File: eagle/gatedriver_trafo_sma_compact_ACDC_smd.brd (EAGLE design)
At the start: 108 x 108 mm, 60 parts, among them K1 G5V-2, X4 BU-SMA-V

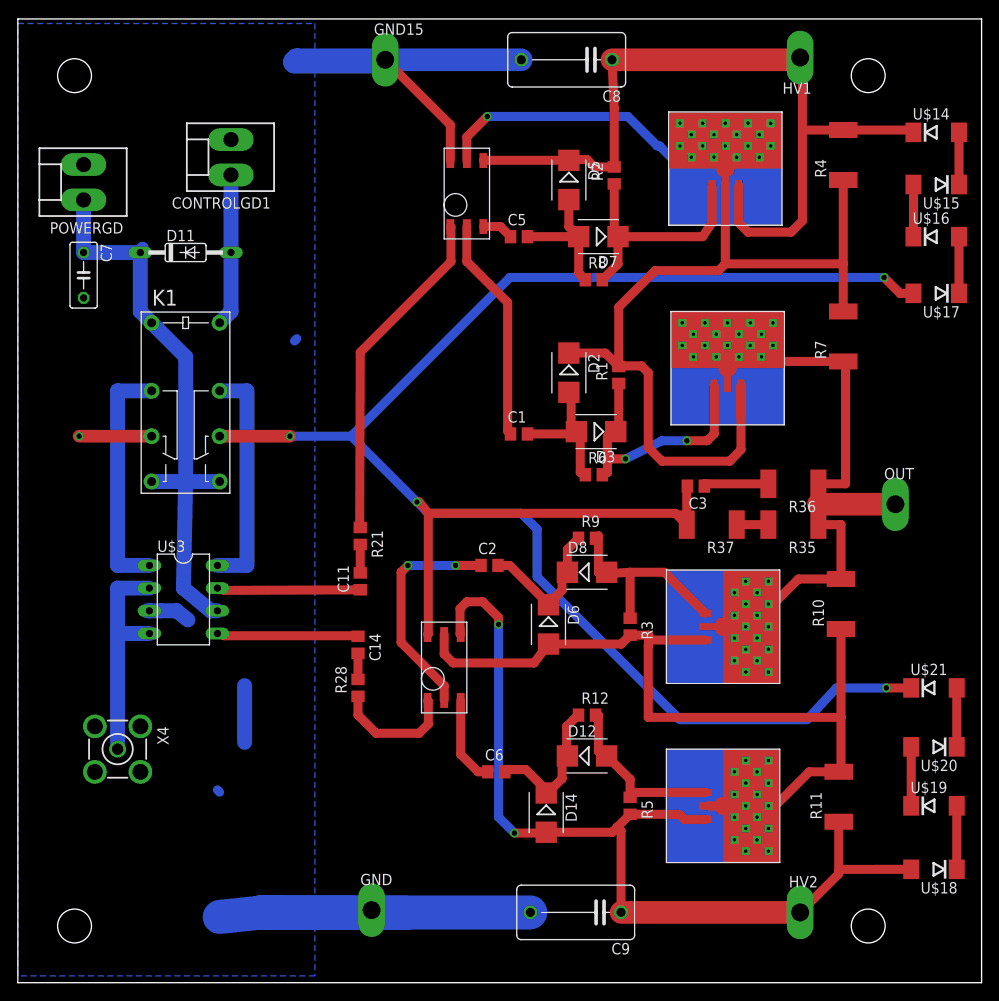
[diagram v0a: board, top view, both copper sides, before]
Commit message: Heatsink, CTIA code
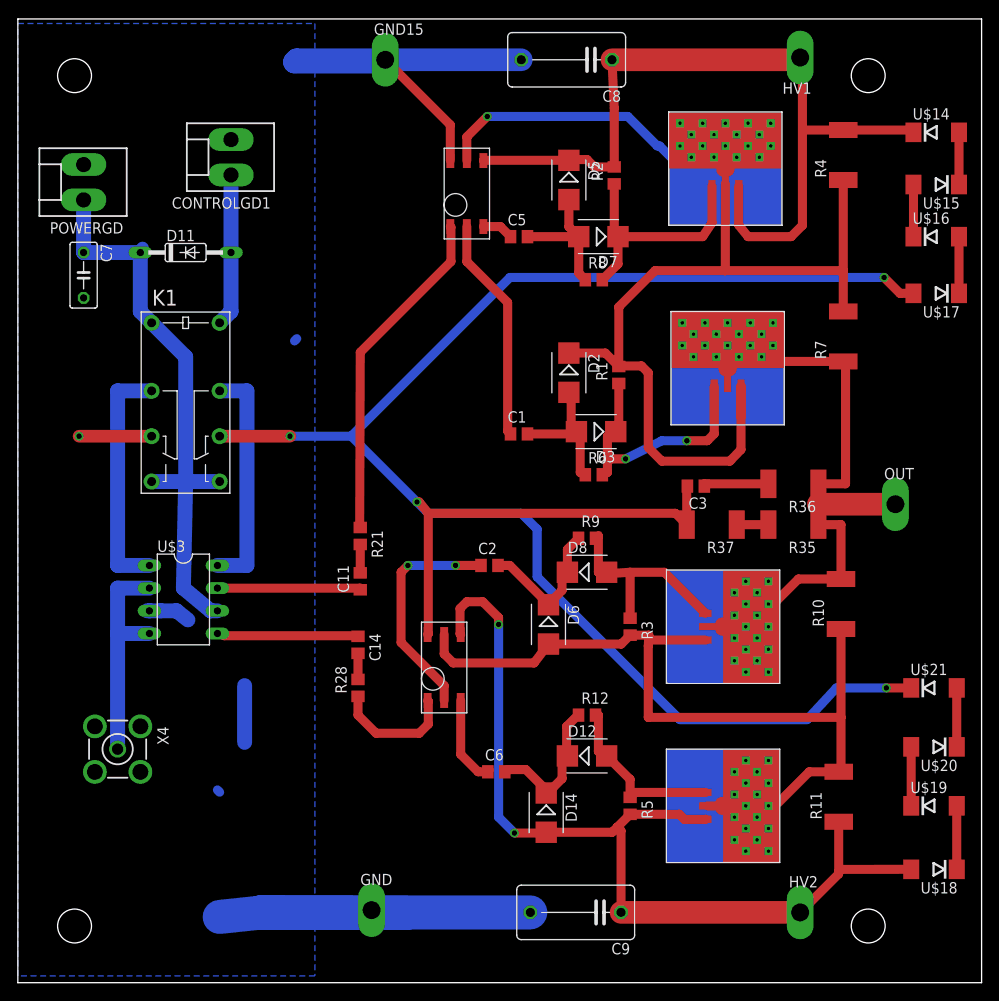
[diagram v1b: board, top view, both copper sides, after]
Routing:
- net N$20: track 70.1 -> 65.3 mm
- net N$6: track 91.4 -> 92.3 mm
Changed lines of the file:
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@@
 <contactref element="U$3" pad="7"/>
 <contactref element="C11" pad="1"/>
-<wire x1="23.114" y1="43.942" x2="22.352" y2="44.196" width="1.016" layer="1"/>
-<wire x1="23.114" y1="43.942" x2="38.608" y2="44.008" width="1.016" layer="1"/>
-<wire x1="38.608" y1="44.008" x2="38.354" y2="44.008" width="1.016" layer="1"/>
+<wire x1="22.352" y1="44.196" x2="38.354" y2="44.196" width="1.016" layer="1"/>
+<wire x1="38.354" y1="44.196" x2="38.354" y2="44.008" width="1.016" layer="1"/>
 </signal>
 <signal name="N$4">
@@
 <wire x1="61.722" y1="92.116" x2="52.1745" y2="92.116" width="1.016" layer="1"/>
 <wire x1="52.1745" y1="92.116" x2="52.1462" y2="92.0877" width="1.016" layer="1"/>
-<wire x1="80.747" y1="89.205" x2="80.747" y2="85.115" width="1.016" layer="1"/>
-<wire x1="80.747" y1="85.115" x2="81.788" y2="84.074" width="1.016" layer="1"/>
-<wire x1="81.788" y1="84.074" x2="86.614" y2="84.074" width="1.016" layer="1"/>
-<wire x1="86.614" y1="84.074" x2="87.884" y2="85.344" width="1.016" layer="1"/>
-<wire x1="87.884" y1="85.344" x2="87.884" y2="95.758" width="1.016" layer="1"/>
+<wire x1="80.747" y1="89.205" x2="80.747" y2="84.861" width="1.016" layer="1"/>
+<wire x1="80.747" y1="84.861" x2="81.788" y2="83.566" width="1.016" layer="1"/>
+<wire x1="81.788" y1="83.566" x2="86.614" y2="83.566" width="1.016" layer="1"/>
+<wire x1="86.614" y1="83.566" x2="87.884" y2="84.836" width="1.016" layer="1"/>
+<wire x1="87.884" y1="84.836" x2="87.884" y2="95.758" width="1.016" layer="1"/>
 <wire x1="87.884" y1="95.758" x2="87.884" y2="103.124" width="1.016" layer="1"/>
 <wire x1="87.884" y1="103.124" x2="87.63" y2="103.378" width="1.016" layer="1"/>
@@
 <wire x1="50.292" y1="92.0877" x2="50.292" y2="94.742" width="1.016" layer="1"/>
 <wire x1="50.292" y1="94.742" x2="52.578" y2="97.028" width="1.016" layer="1"/>
-<wire x1="92.456" y1="89.91" x2="92.456" y2="80.518" width="1.016" layer="1"/>
-<wire x1="92.456" y1="80.518" x2="92.456" y2="75.19" width="1.016" layer="1"/>
-<wire x1="79.248" y1="89.459" x2="79.248" y2="80.518" width="1.016" layer="1"/>
-<wire x1="79.248" y1="80.518" x2="92.456" y2="80.518" width="1.016" layer="1"/>
+<wire x1="92.456" y1="89.91" x2="92.456" y2="79.756" width="1.016" layer="1"/>
+<wire x1="92.456" y1="79.756" x2="92.456" y2="75.19" width="1.016" layer="1"/>
+<wire x1="79.248" y1="89.459" x2="79.248" y2="79.756" width="1.016" layer="1"/>
+<wire x1="79.248" y1="79.756" x2="92.456" y2="79.756" width="1.016" layer="1"/>
 <wire x1="71.882" y1="93.726" x2="71.628" y2="93.726" width="1.016" layer="16"/>
 <wire x1="71.628" y1="93.726" x2="68.326" y2="97.028" width="1.016" layer="16"/>
@@
 <wire x1="67.31" y1="69.022" x2="67.31" y2="75.692" width="1.016" layer="1"/>
 <wire x1="67.31" y1="75.692" x2="71.374" y2="79.756" width="1.016" layer="1"/>
-<wire x1="71.374" y1="79.756" x2="78.486" y2="79.756" width="1.016" layer="1"/>
-<wire x1="78.486" y1="79.756" x2="79.248" y2="80.518" width="1.016" layer="1"/>
+<wire x1="71.374" y1="79.756" x2="79.248" y2="79.756" width="1.016" layer="1"/>
 <wire x1="81.001" y1="66.853" x2="81.001" y2="59.715" width="1.016" layer="1"/>
 <wire x1="81.001" y1="59.715" x2="79.756" y2="58.42" width="1.016" layer="1"/>
@@
 <contactref element="U$2" pad="C"/>
 <contactref element="U$2" pad="C@1"/>
-<wire x1="79.934" y1="39.878" x2="81.500034375" y2="39.280915625" width="1.016" layer="1"/>
-<wire x1="81.500034375" y1="39.280915625" x2="84.398" y2="38.176" width="1.016" layer="1"/>
 <wire x1="92.202" y1="45.218" x2="87.43711875" y2="45.218" width="1.016" layer="1"/>
 <wire x1="87.43711875" y1="45.218" x2="81.500034375" y2="39.280915625" width="1.016" layer="1"/>
@@
 <wire x1="98.298" y1="53.594" x2="89.668" y2="53.594" width="2.54" layer="1"/>
 <wire x1="80.264" y1="69.59" x2="79.502" y2="67.107" width="0" layer="19" extent="1-1"/>
+<wire x1="79.934" y1="39.878" x2="81.500034375" y2="39.280915625" width="0" layer="19" extent="1-1"/>
 <wire x1="77.267" y1="39.878" x2="79.934" y2="39.878" width="0" layer="19" extent="1-1"/>
 </signal>
